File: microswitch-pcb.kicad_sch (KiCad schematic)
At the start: 10 parts, among them J1 Conn_01x06_Socket, U1 D2F-L3, U3 1N4148W_C81598

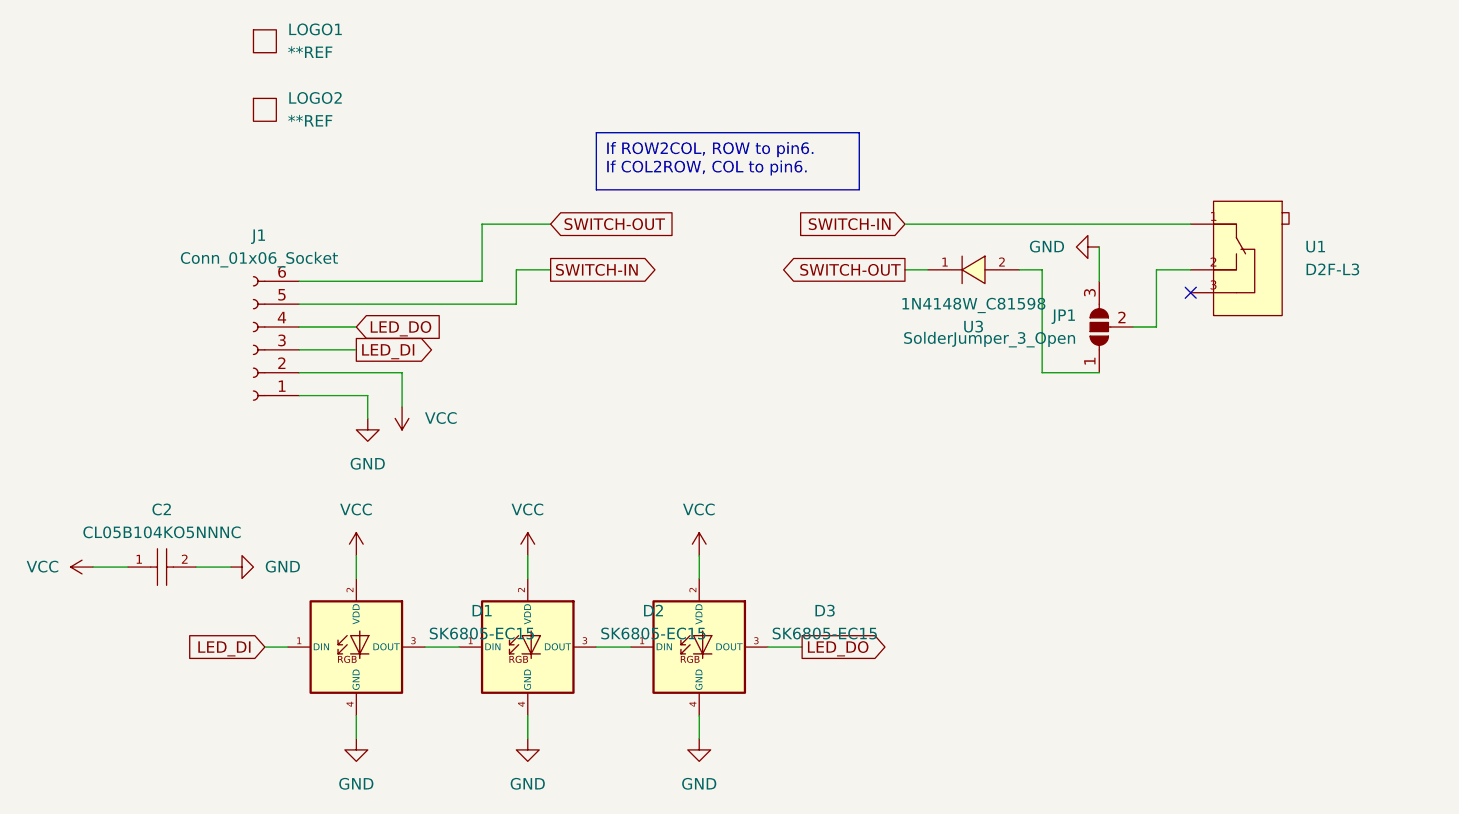
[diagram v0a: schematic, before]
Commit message: adding readme
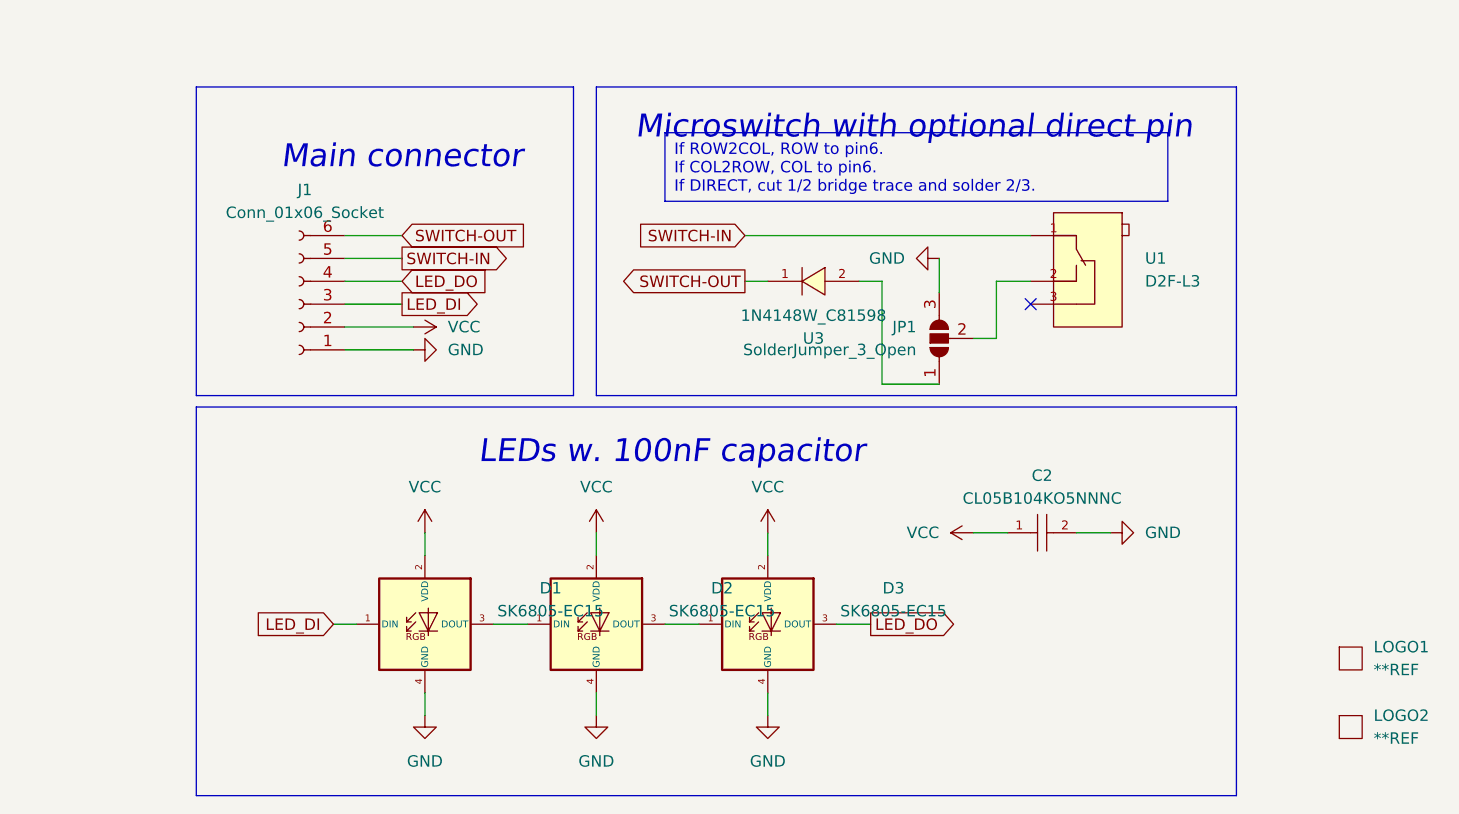
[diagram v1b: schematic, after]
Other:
- note added: "LEDs w. 100nF capacitor"
- note added: "Main connector"
- note added: "Microswitch with optional direct pin"
- moved on the sheet: C2, D1, D2, D3, J1, JP1, LOGO1, LOGO2, U1, U3
